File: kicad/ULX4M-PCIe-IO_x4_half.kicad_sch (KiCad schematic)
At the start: 68 parts, among them J10 FCR684205R, J11 OLED, J12 641737-1, J13 39-30-0060, J14 LM7805_EN, J15 POE, J16 Barrel_Jack, J17 JTAG, J3 SFP+, J4 SFP+, J5 HAT, J6 EXT_USB, J7 Micro_SD_Card_CD, J8 Board_To_Board, J9 FCR684205T, SW1 SW_DIP_x08, SW2 SW_DIP_x08, U10 TPD4E02B04DQA, U11 TPD4E02B04DQA, U12 TPD4E02B04DQA, U13 AT24CS32-SSHM, U14 LM78M05_TO252, U9 TPD4E02B04DQA

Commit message: finalising connections
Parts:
- added AE3: EXT_SERDES_CLK_REF, Connector_Coaxial:SMA_Amphenol_132291-12_Vertical, symbol Device:Antenna_Dipole
- added J18: I2C_to_ID, Connector_PinHeader_2.54mm:PinHeader_2x02_P2.54mm_Vertical, symbol Connector_Generic:Conn_02x02_Odd_Even
- added J19: PCIe_JTAG, Connector_PinHeader_2.54mm:PinHeader_2x04_P2.54mm_Vertical, symbol Connector_Generic:Conn_02x04_Odd_Even
- added J20: PCIe_I2C, Connector_PinHeader_2.54mm:PinHeader_2x02_P2.54mm_Vertical, symbol Connector_Generic:Conn_02x02_Odd_Even
- added J21: PCIe_1X_4X, Connector_PinHeader_2.54mm:PinHeader_2x02_P2.54mm_Vertical, symbol Connector_Generic:Conn_02x02_Odd_Even
- added R23: R220, Resistor_SMD:R_0603_1608Metric, symbol Device:R_Small
- added R24, R27, R28, R29, R46, R47, R48, R49, R50: 4K7, Resistor_SMD:R_0603_1608Metric, symbol Device:R_Small
- added R30, R31, R32, R33, R34, R35, R36, R37, R38, R39, R40, R41, R42, R43, R44, R45: 0R, Resistor_SMD:R_0603_1608Metric, symbol Device:R_Small
- FB1, FB2: footprint (none) -> Inductor_SMD:L_0603_1608Metric
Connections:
- net +12V: now also J15.2 (Pin_2), J15.4 (Pin_4)
- net +3.3V: now also J10.3 (VCC), J11.2 (Pin_2), J9.2 (VCC), R24.1, R27.1, R28.1, R29.1, R46.2, R47.2, R48.2, R49.2, R50.2
- net +5V: now also D1.1 (VDD), D2.1 (VDD), D3.1 (VDD), D4.1 (VDD), D5.1 (VDD), D6.1 (VDD), J6.1 (Pin_1), J6.2 (Pin_2)
- net GND: now also D1.3 (VSS), D2.3 (VSS), D3.3 (VSS), D4.3 (VSS), D5.3 (VSS), D6.3 (VSS), J10.2 (GND), J11.1 (Pin_1), J15.1 (Pin_1), J15.3 (Pin_3), J6.7 (Pin_7), J6.8 (Pin_8), J9.1 (GND), SW1.10, SW1.11, SW1.12, SW1.13, SW1.14, SW1.15, SW1.16, SW1.9, SW2.10, SW2.11, SW2.12, SW2.13, SW2.14, SW2.15, SW2.16, SW2.9, U10.3 (G), U10.8 (G), U9.3 (G), U9.8 (G)
- net GPIO12: now also J19.4 (Pin_4)
- net GPIO16: now also J19.6 (Pin_6)
- net GPIO20: now also J19.2 (Pin_2)
- net GPIO21: now also J19.8 (Pin_8)
- net ID_SC: now also J18.1 (Pin_1)
- net ID_SD: now also J18.3 (Pin_3)
- net PER2_N: now also R35.2, R40.2
- net PER2_P: now also R34.2, R41.2
- net PER3_N: now also R32.2, R38.2
- net PER3_P: now also R33.2, R39.2
- net PET2_N: now also R37.2, R44.2
- net PET2_P: now also R36.2, R45.2
- net PET3_N: now also R30.2, R42.2
- net PET3_P: now also R31.2, R43.2
- net SCL0: now also J18.2 (Pin_2), J20.2 (Pin_2)
- net SDA0: now also J18.4 (Pin_4), J20.4 (Pin_4)
- net SD_CMD: now also R50.1
- net SD_DAT0: now also R46.1
- net SD_DAT1: now also R47.1
- net SD_DAT2: now also R48.1
- net SD_DAT3: now also R49.1
- net SFP0_MOD_ABS: now also R27.2
- net SFP0_RX_N: now also U9.2 (IO2), R36.1
- net SFP0_RX_P: now also U9.1 (IO1), R37.1
- net SFP0_TX_N: now also U9.5 (IO4), R34.1
- net SFP0_TX_P: now also U9.4 (IO3), R35.1
- net SFP1_MOD_ABS: now also R24.2
- net SFP1_RX_N: now also U10.2 (IO2), R32.1
- net SFP1_RX_P: now also U10.1 (IO1), R33.1
- net SFP1_TX_N: now also U10.5 (IO4), R30.1
- net SFP1_TX_P: now also U10.4 (IO3), R31.1
- net SMCLK: now also J20.1 (Pin_1)
- net SMDAT: now also J20.3 (Pin_3)
- net TCK: now also J19.1 (Pin_1)
- net TDI: now also J19.3 (Pin_3)
- net TDO: now also J19.5 (Pin_5)
- net TMS: now also J19.7 (Pin_7)
- net ~{PRSNT1}: now also J21.2 (Pin_2), J21.4 (Pin_4)
- net ~{PRSNT2x1}: now also J21.1 (Pin_1)
- net ~{PRSNT2x4}: now also J21.3 (Pin_3)
- net CAM1_D0_P: now reaches SW2.1
- net CAM1_D0_N: now reaches SW2.2
- net CAM1_D1_P: now reaches SW2.3
- net CAM1_D1_N: now reaches SW2.4
- net CAM0_D0_P: now reaches SW1.1
- net CAM0_D0_N: now reaches SW1.2
- net CAM0_D1_P: now reaches SW1.3
- net CAM0_D1_N: now reaches SW1.4
- net EXT_CLK_REF1_P: now reaches AE1.1
- net EXT_CLK_REF1_N: now reaches AE1.2
- net EXT_CLK_REF2_P: now reaches AE2.1
- net EXT_CLK_REF2_N: now reaches AE2.2
- net OLED_BL: now reaches J3.2 (TX_FAULT), R20.2
- net OLED_BL: now also J11.8 (Pin_8)
- net RS0: now reaches J3.7 (RS0)
- net RS0: now also J4.7 (RS0), R28.2
- net OLED_CS: now reaches J3.8 (RX_LOS), R19.2
- net OLED_CS: now also J11.7 (Pin_7)
- net RS1: now reaches J3.9 (RS1)
- net RS1: now also J4.9 (RS1), R29.2
- net TX_FAULT_1: now reaches J4.2 (TX_FAULT), R22.2
- net RX_LOS_1: now reaches J4.8 (RX_LOS), R21.2
- net USB_ID: now reaches J6.10 (Pin_10)
- net D+: now reaches J6.3 (Pin_3)
- net D+: now also J6.4 (Pin_4)
- net D-: now reaches J6.5 (Pin_5)
- net D-: now also J6.6 (Pin_6)
- net at D2.2 (DOUT): now also D3.4 (DIN)
- net at D2.4 (DIN): now also D1.2 (DOUT)
- net SPDIF_IN: now reaches J9.3 (VIN)
- net at D3.2 (DOUT): now also D4.4 (DIN)
- net at D5.2 (DOUT): now also D6.4 (DIN)
- net at D5.4 (DIN): now also D4.2 (DOUT)
- net OLED_CLK: now reaches J11.3 (Pin_3)
- net OLED_MOSI: now reaches J11.4 (Pin_4)
- net OLED_RES: now reaches J11.5 (Pin_5)
- net OLED_DC: now reaches J11.6 (Pin_6)
- net SPDIF_OUT: now reaches J10.1 (VOUT)
- net at D1.4 (DIN): now also R23.1
- new net EXT__SER_CLK_REF_N: AE3.2
- new net EXT__SER_CLK_REF_P: AE3.1
- new net PER2_PCIe_N: R40.1
- new net PER2_PCIe_P: R41.1
- new net PER3_PCIe_N: R38.1
- new net PER3_PCIe_P: R39.1
- new net PET2_PCIe_N: R44.1
- new net PET2_PCIe_P: R45.1
- new net PET3_PCIe_N: R42.1
- new net PET3_PCIe_P: R43.1
- new net RGB_DATA: R23.2
- no-connect marks 0 -> 1
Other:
- sheet CM4_module ports: added CAM0_C_N, CAM0_C_P, CAM0_D0_N, CAM0_D0_P, CAM0_D1_N, CAM0_D1_P, CAM1_C_N, CAM1_C_P, CAM1_D0_N, CAM1_D0_P, CAM1_D1_N, CAM1_D1_P, Camera_GPIO, DSI0_C_N, DSI0_C_P, DSI0_D0_N, DSI0_D0_P, DSI0_D1_N, DSI0_D1_P, DSI1_C_S1_N, DSI1_C_S1_P, DSI1_D0_S5_N, DSI1_D0_S5_P, DSI1_D1_S7_N, DSI1_D1_S7_P, DSI1_D2_N, DSI1_D2_P, DSI1_D3_N, DSI1_D3_P, ETH0_N, ETH0_P, ETH1_N, ETH1_P, ETH2_N, ETH2_P, ETH3_N, ETH3_P, GPDI1_CEC_PU, GPDI1_HP_PD, GPDI1_SCL_5VPU, GPDI1_SDA_5VPU, PCIe_CLK_N, PCIe_CLK_P, PCIe_CLK_nREQ, PCIe_RX_N, PCIe_RX_P, PCIe_TX_N, PCIe_TX_P, PCIe_nRST, SD_PWR_ON, USB2_N, USB2_P, USB_OTG_ID; removed none
- moved on the sheet: AE1, AE2, C12, C13, C14, C15, D1, D2, D3, D4, D5, D6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

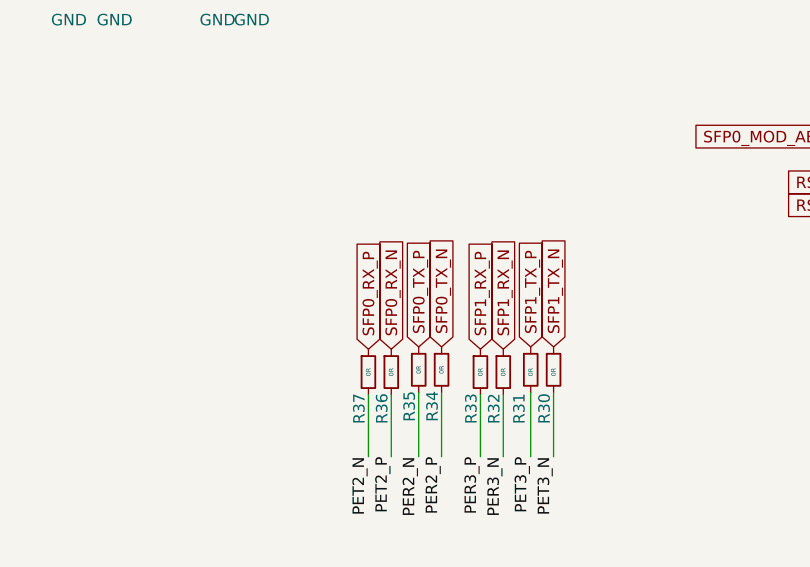
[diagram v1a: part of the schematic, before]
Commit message: Routing PCIe
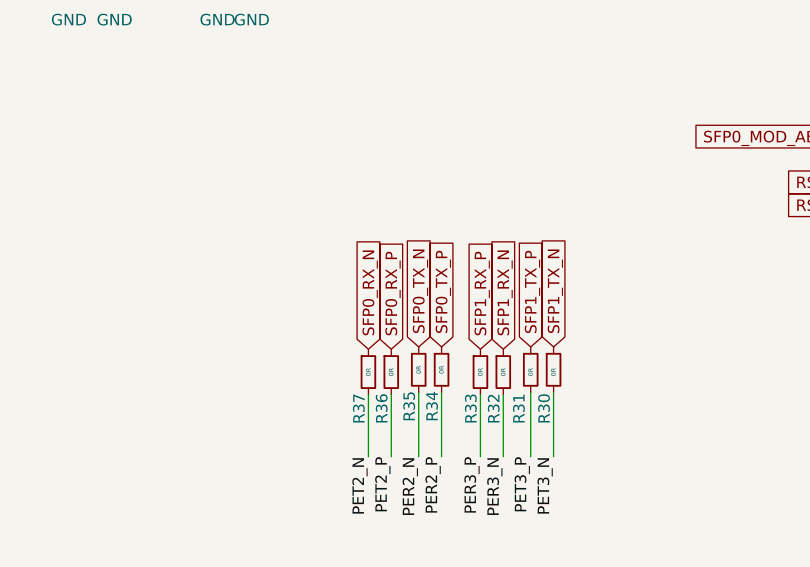
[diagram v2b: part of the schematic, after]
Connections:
- net SFP0_RX_N: now also R37.1; no longer R36.1
- net SFP0_RX_P: now also R36.1; no longer R37.1
- net SFP0_TX_N: now also R35.1; no longer R34.1
- net SFP0_TX_P: now also R34.1; no longer R35.1
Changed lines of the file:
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@@
     )
   )
-  (global_label "SFP0_RX_N" (shape input) (at -144.526 -78.486 90) (fields_autoplaced)
+  (global_label "SFP0_RX_P" (shape input) (at -144.526 -78.486 90) (fields_autoplaced)
     (effects (font (size 1.27 1.27)) (justify left))
     (property "Intersheetrefs" "${INTERSHEET_REFS}" (at -142.6908 -78.486 90)
@@
     )
   )
-  (global_label "SFP0_TX_P" (shape input) (at -141.478 -78.74 90) (fields_autoplaced)
+  (global_label "SFP0_TX_N" (shape input) (at -141.478 -78.74 90) (fields_autoplaced)
     (effects (font (size 1.27 1.27)) (justify left))
     (property "Intersheetrefs" "${INTERSHEET_REFS}" (at -139.6428 -78.74 90)
@@
     )
   )
-  (global_label "SFP0_TX_N" (shape input) (at -138.938 -78.74 90) (fields_autoplaced)
+  (global_label "SFP0_TX_P" (shape input) (at -138.938 -78.74 90) (fields_autoplaced)
     (effects (font (size 1.27 1.27)) (justify left))
     (property "Intersheetrefs" "${INTERSHEET_REFS}" (at -137.1028 -78.74 90)
@@
     )
   )
-  (global_label "SFP0_RX_P" (shape input) (at -147.066 -78.486 90) (fields_autoplaced)
+  (global_label "SFP0_RX_N" (shape input) (at -147.066 -78.486 90) (fields_autoplaced)
     (effects (font (size 1.27 1.27)) (justify left))
     (property "Intersheetrefs" "${INTERSHEET_REFS}" (at -145.2308 -78.486 90)
